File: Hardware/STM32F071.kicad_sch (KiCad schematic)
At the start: 12 parts, among them J1 USB_C_Receptacle_USB2.0_16P, U1 STM32C071K8Tx, U2 USBLC6-2P6, U4 TPS5430

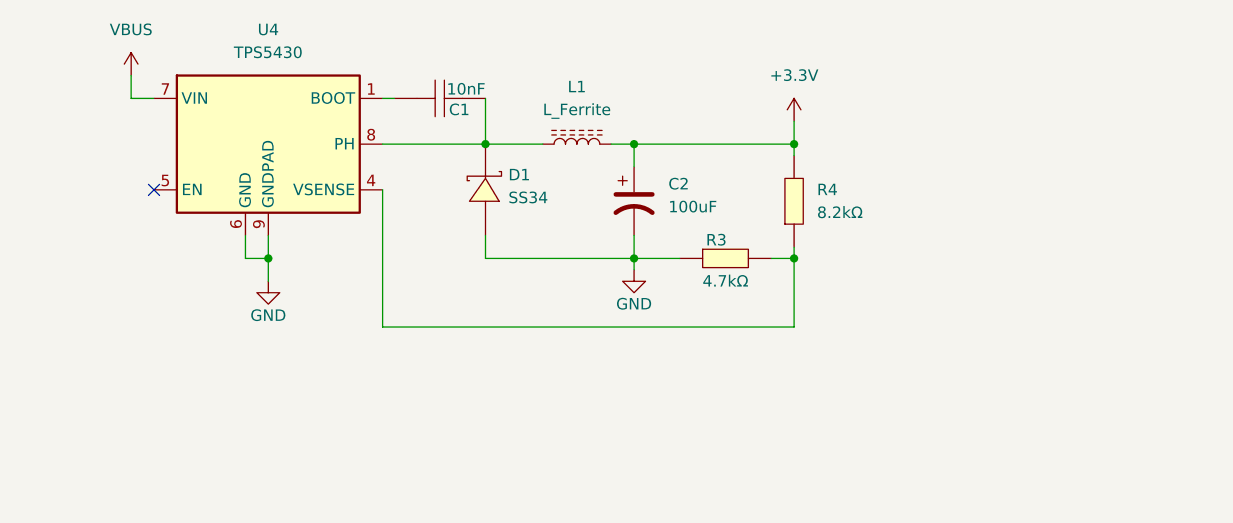
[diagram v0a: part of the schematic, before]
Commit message: More work on power supply
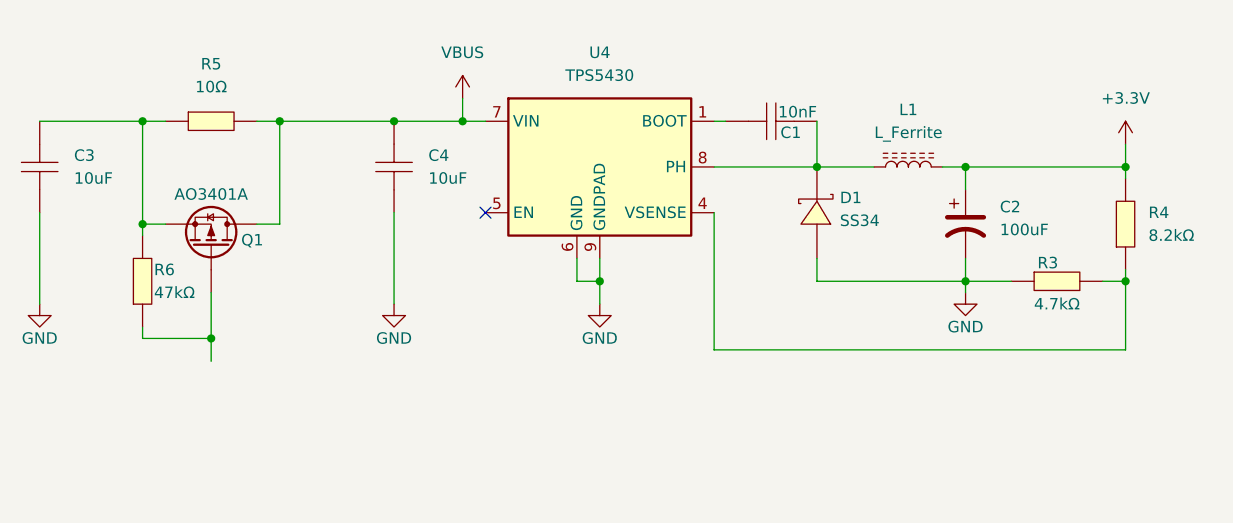
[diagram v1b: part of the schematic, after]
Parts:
- added C3, C4: 10uF, jlcbasic:C1206, symbol jlcbasic:10uF-1206
- added Q1: AO3401A, jlcbasic:SOT-23_L2.9-W1.3-P1.90-LS2.4-BR, symbol jlcbasic:AO3401A
- added R5: 10Ω, jlcbasic:R0805_NEW, symbol jlcbasic:10Ω-0805
- added R6: 47kΩ, jlcbasic:R0805, symbol jlcbasic:47kΩ-0805
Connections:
- net GND: now also C3.1, C4.1
- net VBUS: now also C4.2, Q1.D, R5.2
- new net: C3.2, Q1.S, R5.1, R6.2
- new net: Q1.G, R6.1
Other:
- moved on the sheet: C1, C2, D1, L1, R3, R4, U4
